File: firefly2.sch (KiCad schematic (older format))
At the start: 16 parts, among them J1 10118194-0001LF, P2 CONN_01X03, P3 CONN_01X04, P4 CONN_01X05, P5 CONN_01X01, U1 SAM_D11C, U2 RFM69CW, U3 MIC5504

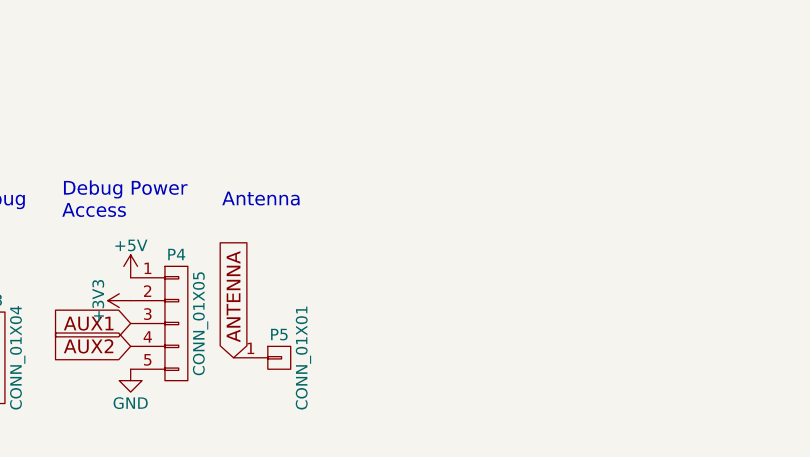
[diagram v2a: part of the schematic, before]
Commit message: Finish routing the board
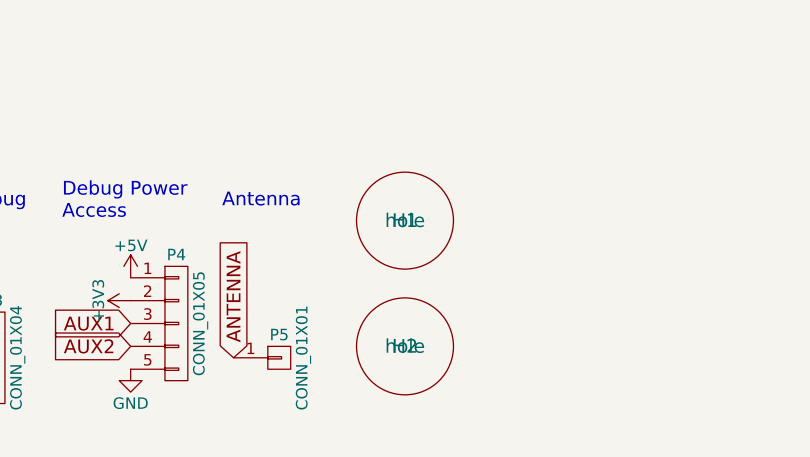
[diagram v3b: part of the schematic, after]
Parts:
- added H1, H2: hole, homebrew:hole-m2.5, symbol hole
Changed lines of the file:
@@
 Off board LED
 $Comp
-L +3V3 #PWR01
+L +3V3 #PWR1
 U 1 1 5A5421BD
 P 1000 1250
-F 0 "#PWR01" H 1000 1100 50  0001 C CNN
+F 0 "#PWR1" H 1000 1100 50  0001 C CNN
 F 1 "+3V3" H 1000 1390 50  0000 C CNN
 F 2 "" H 1000 1250 50  0000 C CNN
@@
 $EndComp
 $Comp
-L +5V #PWR02
+L +5V #PWR5
 U 1 1 5A54225C
 P 2650 7350
-F 0 "#PWR02" H 2650 7200 50  0001 C CNN
+F 0 "#PWR5" H 2650 7200 50  0001 C CNN
 F 1 "+5V" H 2650 7490 50  0000 C CNN
 F 2 "" H 2650 7350 50  0000 C CNN
@@
 $EndComp
 $Comp
-L GND #PWR03
+L GND #PWR6
 U 1 1 5A542285
 P 2650 7550
-F 0 "#PWR03" H 2650 7300 50  0001 C CNN
+F 0 "#PWR6" H 2650 7300 50  0001 C CNN
 F 1 "GND" H 2650 7400 50  0000 C CNN
 F 2 "" H 2650 7550 50  0000 C CNN
@@
 ARM\nSerial Wire Debug
 $Comp
-L +3V3 #PWR04
+L +3V3 #PWR7
 U 1 1 5A54243D
 P 3550 7250
-F 0 "#PWR04" H 3550 7100 50  0001 C CNN
+F 0 "#PWR7" H 3550 7100 50  0001 C CNN
 F 1 "+3V3" H 3550 7390 50  0000 C CNN
 F 2 "" H 3550 7250 50  0000 C CNN
@@
 $EndComp
 $Comp
-L GND #PWR05
+L GND #PWR8
 U 1 1 5A542459
 P 3550 7550
-F 0 "#PWR05" H 3550 7300 50  0001 C CNN
+F 0 "#PWR8" H 3550 7300 50  0001 C CNN
 F 1 "GND" H 3550 7400 50  0000 C CNN
 F 2 "" H 3550 7550 50  0000 C CNN
@@
 	3550 7450 3250 7450
 $Comp
-L +5V #PWR06
+L +5V #PWR3
 U 1 1 5A5424FD
 P 2000 7250
-F 0 "#PWR06" H 2000 7100 50  0001 C CNN
+F 0 "#PWR3" H 2000 7100 50  0001 C CNN
 F 1 "+5V" H 2000 7390 50  0000 C CNN
 F 2 "" H 2000 7250 50  0000 C CNN
@@
 $EndComp
 $Comp
-L GND #PWR07
+L GND #PWR4
 U 1 1 5A542519
 P 2000 7450
-F 0 "#PWR07" H 2000 7200 50  0001 C CNN
+F 0 "#PWR4" H 2000 7200 50  0001 C CNN
 F 1 "GND" H 2000 7300 50  0000 C CNN
 F 2 "" H 2000 7450 50  0000 C CNN
@@
 	850  7350 1000 7350
 $Comp
-L GND #PWR08
+L GND #PWR12
 U 1 1 5A54267D
 P 4350 7450
-F 0 "#PWR08" H 4350 7200 50  0001 C CNN
+F 0 "#PWR12" H 4350 7200 50  0001 C CNN
 F 1 "GND" H 4350 7300 50  0000 C CNN
 F 2 "" H 4350 7450 50  0000 C CNN
@@
 $EndComp
 $Comp
-L +3V3 #PWR09
+L +3V3 #PWR11
 U 1 1 5A54269B
 P 4350 7150
-F 0 "#PWR09" H 4350 7000 50  0001 C CNN
+F 0 "#PWR11" H 4350 7000 50  0001 C CNN
 F 1 "+3V3" H 4350 7290 50  0000 C CNN
 F 2 "" H 4350 7150 50  0000 C CNN
@@
 $EndComp
 $Comp
-L +5V #PWR010
+L +5V #PWR10
 U 1 1 5A5426B9
 P 4350 7050
-F 0 "#PWR010" H 4350 6900 50  0001 C CNN
+F 0 "#PWR10" H 4350 6900 50  0001 C CNN
 F 1 "+5V" H 4350 7190 50  0000 C CNN
 F 2 "" H 4350 7050 50  0000 C CNN
@@
 Debug Power\nAccess
 $Comp
-L GND #PWR011
+L GND #PWR2
 U 1 1 5A542851
 P 1000 1350
-F 0 "#PWR011" H 1000 1100 50  0001 C CNN
+F 0 "#PWR2" H 1000 1100 50  0001 C CNN
 F 1 "GND" H 1000 1200 50  0000 C CNN
 F 2 "" H 1000 1350 50  0000 C CNN
@@
 $EndComp
 $Comp
-L GND #PWR012
+L GND #PWR13
 U 1 1 5A542675
 P 5500 1900
-F 0 "#PWR012" H 5500 1650 50  0001 C CNN
+F 0 "#PWR13" H 5500 1650 50  0001 C CNN
 F 1 "GND" H 5500 1750 50  0000 C CNN
 F 2 "" H 5500 1900 50  0000 C CNN
@@
 $EndComp
 $Comp
-L GND #PWR013
+L GND #PWR14
 U 1 1 5A542695
 P 5500 2100
-F 0 "#PWR013" H 5500 1850 50  0001 C CNN
+F 0 "#PWR14" H 5500 1850 50  0001 C CNN
 F 1 "GND" H 5500 1950 50  0000 C CNN
 F 2 "" H 5500 2100 50  0000 C CNN
@@
 $EndComp
 $Comp
-L +5V #PWR014
+L +5V #PWR15
 U 1 1 5A543862
 P 7150 850
-F 0 "#PWR014" H 7150 700 50  0001 C CNN
+F 0 "#PWR15" H 7150 700 50  0001 C CNN
 F 1 "+5V" H 7150 990 50  0000 C CNN
 F 2 "" H 7150 850 50  0000 C CNN
@@
 $EndComp
 $Comp
-L +5V #PWR015
+L +5V #PWR16
 U 1 1 5A54388C
 P 7150 1650
-F 0 "#PWR015" H 7150 1500 50  0001 C CNN
+F 0 "#PWR16" H 7150 1500 50  0001 C CNN
 F 1 "+5V" H 7150 1790 50  0000 C CNN
 F 2 "" H 7150 1650 50  0000 C CNN
@@
 $EndComp
 $Comp
-L +5V #PWR016
+L +5V #PWR17
 U 1 1 5A543915
 P 7150 2450
-F 0 "#PWR016" H 7150 2300 50  0001 C CNN
+F 0 "#PWR17" H 7150 2300 50  0001 C CNN
 F 1 "+5V" H 7150 2590 50  0000 C CNN
 F 2 "" H 7150 2450 50  0000 C CNN
@@
 $EndComp
 $Comp
-L +5V #PWR017
+L +5V #PWR18
 U 1 1 5A543955
 P 7150 3250
-F 0 "#PWR017" H 7150 3100 50  0001 C CNN
+F 0 "#PWR18" H 7150 3100 50  0001 C CNN
 F 1 "+5V" H 7150 3390 50  0000 C CNN
 F 2 "" H 7150 3250 50  0000 C CNN
@@
 $EndComp
 $Comp
-L GND #PWR018
+L GND #PWR19
 U 1 1 5A54397F
 P 8050 1150
-F 0 "#PWR018" H 8050 900 50  0001 C CNN
+F 0 "#PWR19" H 8050 900 50  0001 C CNN
 F 1 "GND" H 8050 1000 50  0000 C CNN
 F 2 "" H 8050 1150 50  0000 C CNN
@@
 $EndComp
 $Comp
-L GND #PWR019
+L GND #PWR20
 U 1 1 5A5439A9
 P 8050 1950
-F 0 "#PWR019" H 8050 1700 50  0001 C CNN
+F 0 "#PWR20" H 8050 1700 50  0001 C CNN
 F 1 "GND" H 8050 1800 50  0000 C CNN
 F 2 "" H 8050 1950 50  0000 C CNN
@@
 $EndComp
 $Comp
-L GND #PWR020
+L GND #PWR21
 U 1 1 5A5439D3
 P 8050 2750
-F 0 "#PWR020" H 8050 2500 50  0001 C CNN
+F 0 "#PWR21" H 8050 2500 50  0001 C CNN
 F 1 "GND" H 8050 2600 50  0000 C CNN
 F 2 "" H 8050 2750 50  0000 C CNN
@@
 $EndComp
 $Comp
-L GND #PWR021
+L GND #PWR22
 U 1 1 5A543A27
 P 8050 3550
-F 0 "#PWR021" H 8050 3300 50  0001 C CNN
+F 0 "#PWR22" H 8050 3300 50  0001 C CNN
 F 1 "GND" H 8050 3400 50  0000 C CNN
 F 2 "" H 8050 3550 50  0000 C CNN
@@
 $EndComp
 $Comp
-L GND #PWR022
+L GND #PWR23
 U 1 1 5A5473E5
 P 9800 1150
-F 0 "#PWR022" H 9800 900 50  0001 C CNN
+F 0 "#PWR23" H 9800 900 50  0001 C CNN
 F 1 "GND" H 9800 1000 50  0000 C CNN
 F 2 "" H 9800 1150 50  0000 C CNN
@@
 $EndComp
 $Comp
-L +5V #PWR023
+L +5V #PWR24
 U 1 1 5A547413
 P 10000 750
-F 0 "#PWR023" H 10000 600 50  0001 C CNN
+F 0 "#PWR24" H 10000 600 50  0001 C CNN
 F 1 "+5V" H 10000 890 50  0000 C CNN
 F 2 "" H 10000 750 50  0000 C CNN
@@
 $EndComp
 $Comp
-L +3V3 #PWR024
+L +3V3 #PWR25
 U 1 1 5A547441
 P 10950 950
-F 0 "#PWR024" H 10950 800 50  0001 C CNN
+F 0 "#PWR25" H 10950 800 50  0001 C CNN
 F 1 "+3V3" H 10950 1090 50  0000 C CNN
 F 2 "" H 10950 950 50  0000 C CNN
@@
 $EndComp
 $Comp
-L GND #PWR025
+L GND #PWR26
 U 1 1 5A547D81
 P 10950 1250
-F 0 "#PWR025" H 10950 1000 50  0001 C CNN
+F 0 "#PWR26" H 10950 1000 50  0001 C CNN
 F 1 "GND" H 10950 1100 50  0000 C CNN
 F 2 "" H 10950 1250 50  0000 C CNN
@@
 Connection ~ 9800 1050
 $Comp
-L +3V3 #PWR026
+L +3V3 #PWR9
 U 1 1 5A54A758
 P 4300 1300
-F 0 "#PWR026" H 4300 1150 50  0001 C CNN
+F 0 "#PWR9" H 4300 1150 50  0001 C CNN
 F 1 "+3V3" H 4300 1440 50  0000 C CNN
 F 2 "" H 4300 1300 50  0000 C CNN
@@
 $EndComp
 NoConn ~ 1000 7450
+$Comp
+L hole H1
+U 1 1 5A5AA266
+P 5550 6800
+F 0 "H1" H 5550 6800 60  0000 C CNN
+F 1 "hole" H 5550 6800 60  0000 C CNN
+F 2 "homebrew:hole-m2.5" H 5550 6800 60  0001 C CNN
+F 3 "" H 5550 6800 60  0000 C CNN
+	1    5550 6800
+	1    0    0    -1
+$EndComp
+$Comp
+L hole H2
+U 1 1 5A5AA2E7
+P 5550 7350
+F 0 "H2" H 5550 7350 60  0000 C CNN
+F 1 "hole" H 5550 7350 60  0000 C CNN
+F 2 "homebrew:hole-m2.5" H 5550 7350 60  0001 C CNN
+F 3 "" H 5550 7350 60  0000 C CNN
+	1    5550 7350
+	1    0    0    -1
+$EndComp
 $EndSCHEMATC
